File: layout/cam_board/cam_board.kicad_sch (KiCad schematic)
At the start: 75 parts, among them J1 Conn_01x04_Pin, J2 USB Connector, J3 BATT_CONNECTOR, J4 LCD conn, J5 Stick conn, SW1 BOOT0, SW2 NRST, SW3 USER, SW4 ON/OFF, U1 STM32F401CCUx, U2 USBLC6-2SC6, U3 M24C16-RMN6TP, U4 AP2112K-3.3, U5 MCP73871-1AA, Y1 ECS-80-18-23B-JTN-TR, Y2 SC32S-7PF20PPM

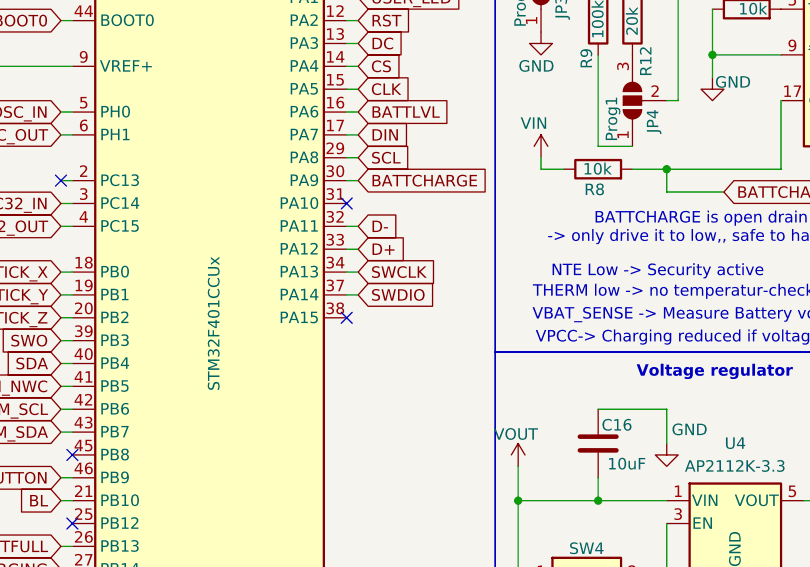
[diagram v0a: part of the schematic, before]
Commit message: Update layout and schematic
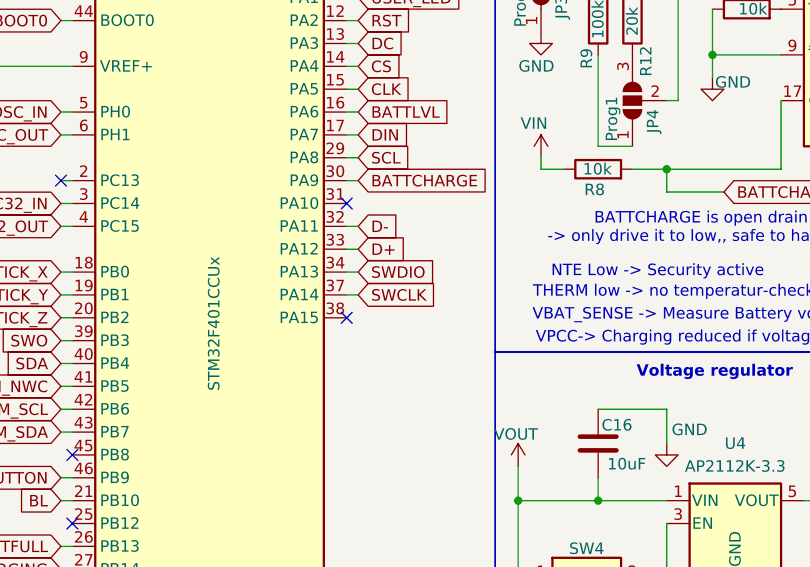
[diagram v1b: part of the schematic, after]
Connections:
- net SWCLK: now also U1.37 (PA14); no longer U1.34 (PA13)
- net SWDIO: now also U1.34 (PA13); no longer U1.37 (PA14)
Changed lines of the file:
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@@
 		)
 	)
-	(global_label "SWDIO"
-		(shape input)
-		(at 156.21 95.25 0)
-		(fields_autoplaced yes)
-		(effects
-			(font
-				(size 1.27 1.27)
-			)
-			(justify left)
-		)
-		(property "Intersheetrefs" "${INTERSHEET_REFS}"
-			(at 165.0614 95.25 0)
-			(effects
-				(font
-					(size 1.27 1.27)
-				)
-				(justify left)
-				(hide yes)
-			)
-		)
-	)
 	(global_label "DC"
 		(shape input)
@@
 		)
 	)
+	(global_label "SWDIO"
+		(shape input)
+		(at 156.21 92.71 0)
+		(fields_autoplaced yes)
+		(effects
+			(font
+				(size 1.27 1.27)
+			)
+			(justify left)
+		)
+		(property "Intersheetrefs" "${INTERSHEET_REFS}"
+			(at 165.0614 92.71 0)
+			(effects
+				(font
+					(size 1.27 1.27)
+				)
+				(justify left)
+				(hide yes)
+			)
+		)
+	)
 	(global_label "D+"
 		(shape input)
@@
 		)
 	)
-	(global_label "SWCLK"
-		(shape input)
-		(at 156.21 92.71 0)
-		(fields_autoplaced yes)
-		(effects
-			(font
-				(size 1.27 1.27)
-			)
-			(justify left)
-		)
-		(property "Intersheetrefs" "${INTERSHEET_REFS}"
-			(at 165.4242 92.71 0)
-			(effects
-				(font
-					(size 1.27 1.27)
-				)
-				(justify left)
-				(hide yes)
-			)
-		)
-	)
 	(global_label "BATTCHARGE"
 		(shape input)
@@
 		)
 	)
+	(global_label "SWCLK"
+		(shape input)
+		(at 156.21 95.25 0)
+		(fields_autoplaced yes)
+		(effects
+			(font
+				(size 1.27 1.27)
+			)
+			(justify left)
+		)
+		(property "Intersheetrefs" "${INTERSHEET_REFS}"
+			(at 165.4242 95.25 0)
+			(effects
+				(font
+					(size 1.27 1.27)
+				)
+				(justify left)
+				(hide yes)
+			)
+		)
+	)
 	(global_label "BATTCHARGING"
 		(shape input)
@@
 	)
 	(symbol
+		(lib_name "+5V_3")
 		(lib_id "power:+5V")
 		(at 250.19 54.61 0)
@@
 	)
 	(symbol
+		(lib_name "+5V_2")
 		(lib_id "power:+5V")
 		(at 228.6 21.59 0)
@@
 	)
 	(symbol
+		(lib_name "+5V_1")
 		(lib_id "power:+5V")
 		(at 187.96 26.67 0)
@@
 	)
 	(symbol
+		(lib_name "SolderJumper_3_Open_1")
 		(lib_id "Jumper:SolderJumper_3_Open")
 		(at 228.6 34.29 180)
